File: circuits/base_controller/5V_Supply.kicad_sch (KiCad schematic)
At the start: 4 parts, among them J6 Barrel_Jack, U3 AMS1117-5.0

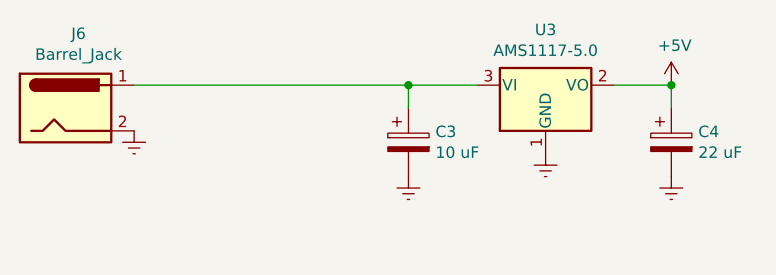
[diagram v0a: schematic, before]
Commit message: Big updates
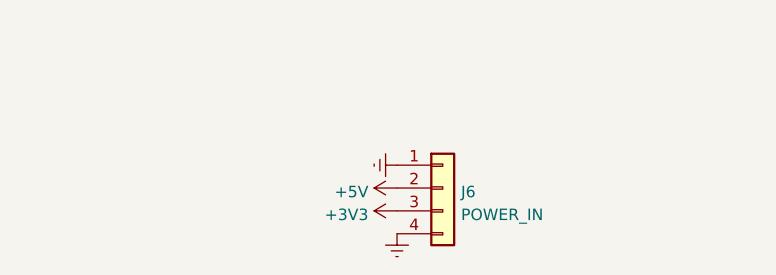
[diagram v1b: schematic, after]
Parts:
- removed C3: 10 uF, Capacitor_THT:CP_Radial_D5.0mm_P2.00mm, symbol base_controller-rescue:CP-Device
- removed C4: 22 uF, Capacitor_THT:CP_Radial_D5.0mm_P2.00mm, symbol base_controller-rescue:CP-Device
- removed J6: Barrel_Jack, Connector_BarrelJack:BarrelJack_Horizontal, symbol Connector:Barrel_Jack
- removed U3: AMS1117-5.0, Package_TO_SOT_SMD:TO-252-3_TabPin4, symbol Regulator_Linear:AMS1117-5.0
- added J6: POWER_IN, Connector_JST:JST_XH_B4B-XH-A_1x04_P2.50mm_Vertical, symbol Connector_Generic:Conn_01x04
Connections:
- net +5V: now also J6.2 (Pin_2)
- net Earth: now also J6.1 (Pin_1), J6.4 (Pin_4)
- new net +3V3: J6.3 (Pin_3)
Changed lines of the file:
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@@
 (kicad_sch (version 20211123) (generator eeschema)
   (paper "A4")
-  (junction (at 148.59 85.09) (diameter 0) (color 0 0 0 0)
-  )
-  (junction (at 119.38 85.09) (diameter 0) (color 0 0 0 0)
-  )
-  (wire (pts (xy 142.24 85.09) (xy 148.59 85.09))
-    (stroke (width 0) (type default) (color 0 0 0 0))
-  )
-  (wire (pts (xy 148.59 85.09) (xy 148.59 87.63))
-    (stroke (width 0) (type default) (color 0 0 0 0))
-  )
-  (wire (pts (xy 88.9 85.09) (xy 119.38 85.09))
-    (stroke (width 0) (type default) (color 0 0 0 0))
-  )
-  (wire (pts (xy 127 85.09) (xy 119.38 85.09))
-    (stroke (width 0) (type default) (color 0 0 0 0))
-  )
-  (wire (pts (xy 119.38 85.09) (xy 119.38 87.63))
-    (stroke (width 0) (type default) (color 0 0 0 0))
-  )
-  (symbol (lib_id "Regulator_Linear:AMS1117-5.0") (at 134.62 85.09 0) (unit 1)
-    (in_bom yes) (on_board yes)
-    (property "Reference" "U3" (id 0) (at 134.62 78.9432 0))
-    (property "Value" "AMS1117-5.0" (id 1) (at 134.62 81.2546 0))
-    (property "Footprint" "Package_TO_SOT_SMD:TO-252-3_TabPin4" (id 2) (at 134.62 80.01 0)
+  (symbol (lib_id "power:Earth") (at 118.11 93.98 270) (unit 1)
+    (in_bom yes) (on_board yes) (fields_autoplaced)
+    (property "Reference" "#PWR021" (id 0) (at 111.76 93.98 0)
       (effects (font (size 1.27 1.27)) hide)
     )
-    (property "Datasheet" "http://www.advanced-monolithic.com/pdf/ds1117.pdf" (id 3) (at 137.16 91.44 0)
+    (property "Value" "Earth" (id 1) (at 114.3 93.98 0)
+      (effects (font (size 1.27 1.27)) hide)
+    )
+    (property "Footprint" "" (id 2) (at 118.11 93.98 0)
+      (effects (font (size 1.27 1.27)) hide)
+    )
+    (property "Datasheet" "~" (id 3) (at 118.11 93.98 0)
+      (effects (font (size 1.27 1.27)) hide)
+    )
+    (pin "1")
+  )
+  (symbol (lib_id "Connector_Generic:Conn_01x04") (at 123.19 96.52 0) (unit 1)
+    (in_bom yes) (on_board yes) (fields_autoplaced)
+    (property "Reference" "J6" (id 0) (at 125.222 96.9553 0)
+      (effects (font (size 1.27 1.27)) (justify left))
+    )
+    (property "Value" "POWER_IN" (id 1) (at 125.222 99.4922 0)
+      (effects (font (size 1.27 1.27)) (justify left))
+    )
+    (property "Footprint" "Connector_JST:JST_XH_B4B-XH-A_1x04_P2.50mm_Vertical" (id 2) (at 123.19 96.52 0)
+      (effects (font (size 1.27 1.27)) hide)
+    )
+    (property "Datasheet" "~" (id 3) (at 123.19 96.52 0)
       (effects (font (size 1.27 1.27)) hide)
     )
@@
     (pin "2")
     (pin "3")
+    (pin "4")
   )
-  (symbol (lib_id "base_controller-rescue:CP-Device") (at 119.38 91.44 0) (unit 1)
-    (in_bom yes) (on_board yes)
-    (property "Reference" "C3" (id 0) (at 122.3772 90.2716 0)
+  (symbol (lib_id "power:+5V") (at 118.11 96.52 90) (unit 1)
+    (in_bom yes) (on_board yes) (fields_autoplaced)
+    (property "Reference" "#PWR022" (id 0) (at 121.92 96.52 0)
+      (effects (font (size 1.27 1.27)) hide)
+    )
+    (property "Value" "+5V" (id 1) (at 114.9351 96.9538 90)
       (effects (font (size 1.27 1.27)) (justify left))
     )
-    (property "Value" "10 uF" (id 1) (at 122.3772 92.583 0)
-      (effects (font (size 1.27 1.27)) (justify left))
-    )
-    (property "Footprint" "Capacitor_THT:CP_Radial_D5.0mm_P2.00mm" (id 2) (at 120.3452 95.25 0)
+    (property "Footprint" "" (id 2) (at 118.11 96.52 0)
       (effects (font (size 1.27 1.27)) hide)
     )
-    (property "Datasheet" "~" (id 3) (at 119.38 91.44 0)
-      (effects (font (size 1.27 1.27)) hide)
-    )
-    (pin "1")
-    (pin "2")
-  )
-  (symbol (lib_id "base_controller-rescue:CP-Device") (at 148.59 91.44 0) (unit 1)
-    (in_bom yes) (on_board yes)
-    (property "Reference" "C4" (id 0) (at 151.5872 90.2716 0)
-      (effects (font (size 1.27 1.27)) (justify left))
-    )
-    (property "Value" "22 uF" (id 1) (at 151.5872 92.583 0)
-      (effects (font (size 1.27 1.27)) (justify left))
-    )
-    (property "Footprint" "Capacitor_THT:CP_Radial_D5.0mm_P2.00mm" (id 2) (at 149.5552 95.25 0)
-      (effects (font (size 1.27 1.27)) hide)
-    )
-    (property "Datasheet" "~" (id 3) (at 148.59 91.44 0)
-      (effects (font (size 1.27 1.27)) hide)
-    )
-    (pin "1")
-    (pin "2")
-  )
-  (symbol (lib_id "power:+5V") (at 148.59 85.09 0) (unit 1)
-    (in_bom yes) (on_board yes)
-    (property "Reference" "#PWR0107" (id 0) (at 148.59 88.9 0)
-      (effects (font (size 1.27 1.27)) hide)
-    )
-    (property "Value" "+5V" (id 1) (at 148.971 80.6958 0))
-    (property "Footprint" "" (id 2) (at 148.59 85.09 0)
-      (effects (font (size 1.27 1.27)) hide)
-    )
-    (property "Datasheet" "" (id 3) (at 148.59 85.09 0)
+    (property "Datasheet" "" (id 3) (at 118.11 96.52 0)
       (effects (font (size 1.27 1.27)) hide)
     )
     (pin "1")
   )
-  (symbol (lib_id "power:Earth") (at 119.38 95.25 0) (unit 1)
-    (in_bom yes) (on_board yes)
-    (property "Reference" "#PWR0108" (id 0) (at 119.38 101.6 0)
+  (symbol (lib_id "power:+3V3") (at 118.11 99.06 90) (unit 1)
+    (in_bom yes) (on_board yes) (fields_autoplaced)
+    (property "Reference" "#PWR023" (id 0) (at 121.92 99.06 0)
       (effects (font (size 1.27 1.27)) hide)
     )
-    (property "Value" "Earth" (id 1) (at 119.38 99.06 0)
+    (property "Value" "+3V3" (id 1) (at 114.935 99.4938 90)
+      (effects (font (size 1.27 1.27)) (justify left))
+    )
+    (property "Footprint" "" (id 2) (at 118.11 99.06 0)
       (effects (font (size 1.27 1.27)) hide)
     )
-    (property "Footprint" "" (id 2) (at 119.38 95.25 0)
-      (effects (font (size 1.27 1.27)) hide)
-    )
-    (property "Datasheet" "~" (id 3) (at 119.38 95.25 0)
+    (property "Datasheet" "" (id 3) (at 118.11 99.06 0)
       (effects (font (size 1.27 1.27)) hide)
     )
     (pin "1")
   )
-  (symbol (lib_id "power:Earth") (at 134.62 92.71 0) (unit 1)
-    (in_bom yes) (on_board yes)
-    (property "Reference" "#PWR0109" (id 0) (at 134.62 99.06 0)
+  (symbol (lib_id "power:Earth") (at 118.11 101.6 0) (unit 1)
+    (in_bom yes) (on_board yes) (fields_autoplaced)
+    (property "Reference" "#PWR024" (id 0) (at 118.11 107.95 0)
       (effects (font (size 1.27 1.27)) hide)
     )
-    (property "Value" "Earth" (id 1) (at 134.62 96.52 0)
+    (property "Value" "Earth" (id 1) (at 118.11 105.41 0)
       (effects (font (size 1.27 1.27)) hide)
     )
-    (property "Footprint" "" (id 2) (at 134.62 92.71 0)
+    (property "Footprint" "" (id 2) (at 118.11 101.6 0)
       (effects (font (size 1.27 1.27)) hide)
     )
-    (property "Datasheet" "~" (id 3) (at 134.62 92.71 0)
+    (property "Datasheet" "~" (id 3) (at 118.11 101.6 0)
       (effects (font (size 1.27 1.27)) hide)
     )
-    (pin "1")
-  )
-  (symbol (lib_id "power:Earth") (at 148.59 95.25 0) (unit 1)
-    (in_bom yes) (on_board yes)
-    (property "Reference" "#PWR0110" (id 0) (at 148.59 101.6 0)
-      (effects (font (size 1.27 1.27)) hide)
-    )
-    (property "Value" "Earth" (id 1) (at 148.59 99.06 0)
-      (effects (font (size 1.27 1.27)) hide)
-    )
-    (property "Footprint" "" (id 2) (at 148.59 95.25 0)
-      (effects (font (size 1.27 1.27)) hide)
-    )
-    (property "Datasheet" "~" (id 3) (at 148.59 95.25 0)
-      (effects (font (size 1.27 1.27)) hide)
-    )
-    (pin "1")
-  )
-  (symbol (lib_id "Connector:Barrel_Jack") (at 81.28 87.63 0) (unit 1)
-    (in_bom yes) (on_board yes)
-    (property "Reference" "J6" (id 0) (at 82.7278 79.375 0))
-    (property "Value" "Barrel_Jack" (id 1) (at 82.7278 81.6864 0))
-    (property "Footprint" "Connector_BarrelJack:BarrelJack_Horizontal" (id 2) (at 82.55 88.646 0)
-      (effects (font (size 1.27 1.27)) hide)
-    )
-    (property "Datasheet" "~" (id 3) (at 82.55 88.646 0)
-      (effects (font (size 1.27 1.27)) hide)
-    )
-    (pin "1")
-    (pin "2")
-  )
-  (symbol (lib_id "power:Earth") (at 88.9 90.17 0) (unit 1)
-    (in_bom yes) (on_board yes)
-    (property "Reference" "#PWR0111" (id 0) (at 88.9 96.52 0)
-      (effects (font (size 1.27 1.27)) hide)
-    )
-    (property "Value" "Earth" (id 1) (at 88.9 93.98 0)
-      (effects (font (size 1.27 1.27)) hide)
-    )
-    (property "Footprint" "" (id 2) (at 88.9 90.17 0)
-      (effects (font (size 1.27 1.27)) hide)
-    )
-    (property "Datasheet" "~" (id 3) (at 88.9 90.17 0)
-      (effects (font (size 1.27 1.27)) hide)
-    )
